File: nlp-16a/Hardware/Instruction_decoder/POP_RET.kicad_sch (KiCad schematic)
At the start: 12 parts

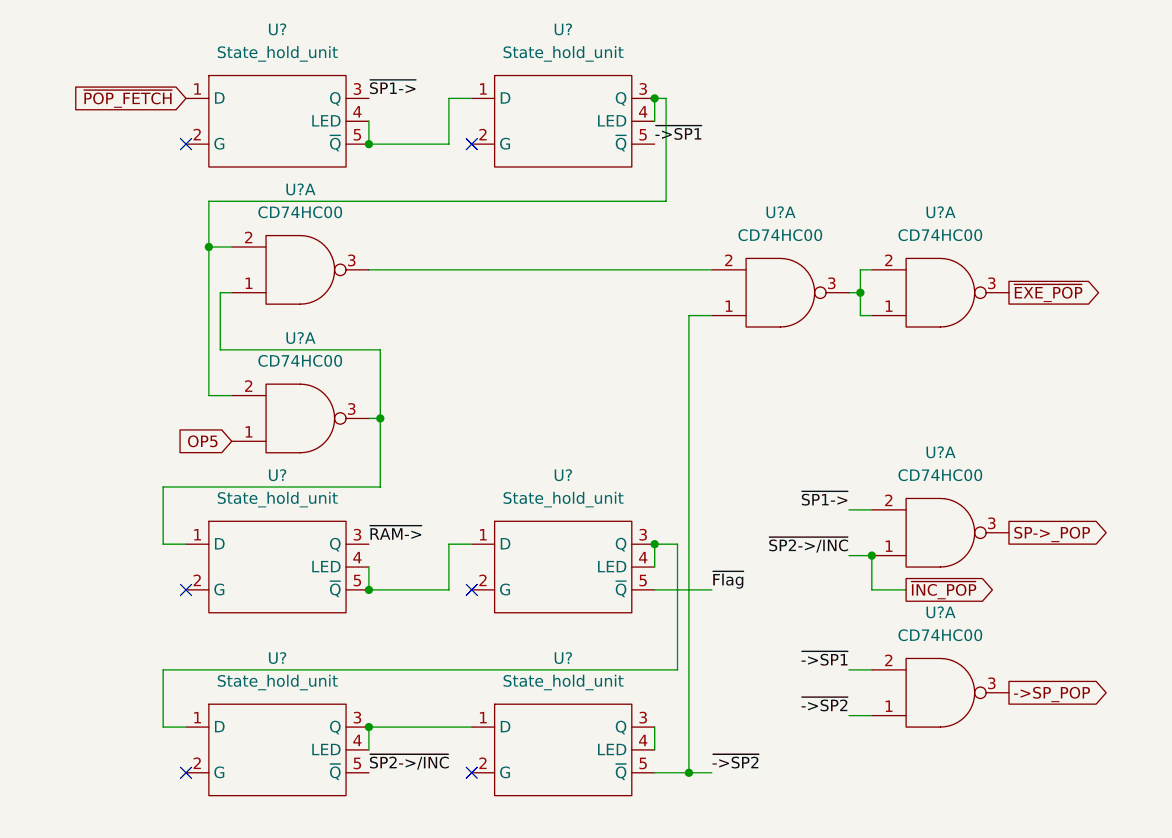
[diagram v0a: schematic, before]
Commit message: 命令デコーダ ロジック部の設計だいたい完了git statusgit statusやったぜ
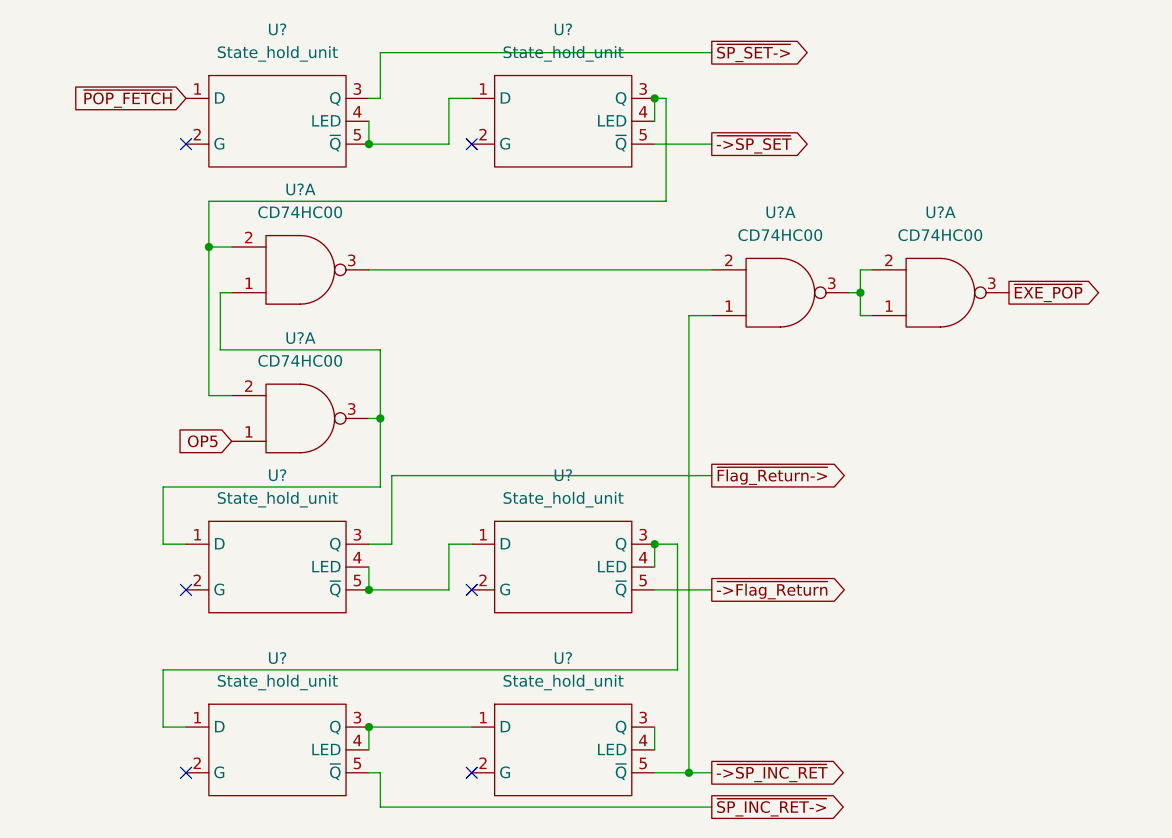
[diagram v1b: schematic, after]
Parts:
- removed U? (x2): CD74HC00, Package_DIP:DIP-14_W7.62mm, symbol CD74HCXX:CD74HC00
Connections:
- net ~{->SP1} renamed ~{->SP_SET}
- net ~{->SP2} renamed ~{->SP_INC_RET}
- net ~{Flag} renamed ~{->Flag_Return}
- net ~{INC_POP} renamed ~{SP_INC_RET->}
- net ~{RAM->} renamed ~{Flag_Return->}
- net ~{SP1->} renamed ~{SP_SET->}
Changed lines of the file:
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@@
   (junction (at 165.1 53.34) (diameter 0) (color 0 0 0 0)
-  )
-  (junction (at 166.37 82.55) (diameter 0) (color 0 0 0 0)
   )
   (junction (at 142.24 31.75) (diameter 0) (color 0 0 0 0)
@@
   (no_connect (at 121.92 86.36))
   (no_connect (at 90.17 106.68))
-  (wire (pts (xy 166.37 82.55) (xy 166.37 86.36))
+  (wire (pts (xy 142.24 36.83) (xy 148.59 36.83))
     (stroke (width 0) (type default) (color 0 0 0 0))
   )
@@
     (stroke (width 0) (type default) (color 0 0 0 0))
   )
+  (wire (pts (xy 113.03 73.66) (xy 148.59 73.66))
+    (stroke (width 0) (type default) (color 0 0 0 0))
+  )
   (wire (pts (xy 146.05 55.88) (xy 148.59 55.88))
     (stroke (width 0) (type default) (color 0 0 0 0))
@@
     (stroke (width 0) (type default) (color 0 0 0 0))
   )
+  (wire (pts (xy 111.76 31.75) (xy 111.76 26.67))
+    (stroke (width 0) (type default) (color 0 0 0 0))
+  )
   (wire (pts (xy 142.24 81.28) (xy 144.78 81.28))
     (stroke (width 0) (type default) (color 0 0 0 0))
@@
     (stroke (width 0) (type default) (color 0 0 0 0))
   )
+  (wire (pts (xy 110.49 31.75) (xy 111.76 31.75))
+    (stroke (width 0) (type default) (color 0 0 0 0))
+  )
   (wire (pts (xy 143.51 43.18) (xy 92.71 43.18))
     (stroke (width 0) (type default) (color 0 0 0 0))
@@
     (stroke (width 0) (type default) (color 0 0 0 0))
   )
+  (wire (pts (xy 111.76 106.68) (xy 111.76 110.49))
+    (stroke (width 0) (type default) (color 0 0 0 0))
+  )
   (wire (pts (xy 142.24 101.6) (xy 142.24 104.14))
     (stroke (width 0) (type default) (color 0 0 0 0))
@@
     (stroke (width 0) (type default) (color 0 0 0 0))
   )
-  (wire (pts (xy 163.83 82.55) (xy 166.37 82.55))
-    (stroke (width 0) (type default) (color 0 0 0 0))
-  )
-  (wire (pts (xy 170.18 86.36) (xy 166.37 86.36))
+  (wire (pts (xy 113.03 81.28) (xy 113.03 73.66))
+    (stroke (width 0) (type default) (color 0 0 0 0))
+  )
+  (wire (pts (xy 111.76 110.49) (xy 148.59 110.49))
     (stroke (width 0) (type default) (color 0 0 0 0))
   )
@@
     (stroke (width 0) (type default) (color 0 0 0 0))
   )
-  (wire (pts (xy 163.83 77.47) (xy 166.37 77.47))
+  (wire (pts (xy 110.49 106.68) (xy 111.76 106.68))
+    (stroke (width 0) (type default) (color 0 0 0 0))
+  )
+  (wire (pts (xy 110.49 81.28) (xy 113.03 81.28))
     (stroke (width 0) (type default) (color 0 0 0 0))
   )
@@
     (stroke (width 0) (type default) (color 0 0 0 0))
   )
+  (wire (pts (xy 111.76 26.67) (xy 148.59 26.67))
+    (stroke (width 0) (type default) (color 0 0 0 0))
+  )
   (wire (pts (xy 90.17 101.6) (xy 87.63 101.6))
     (stroke (width 0) (type default) (color 0 0 0 0))
@@
     (stroke (width 0) (type default) (color 0 0 0 0))
   )
-  (wire (pts (xy 163.83 95.25) (xy 166.37 95.25))
-    (stroke (width 0) (type default) (color 0 0 0 0))
-  )
   (wire (pts (xy 143.51 31.75) (xy 143.51 43.18))
     (stroke (width 0) (type default) (color 0 0 0 0))
@@
     (stroke (width 0) (type default) (color 0 0 0 0))
   )
-  (wire (pts (xy 163.83 100.33) (xy 166.37 100.33))
-    (stroke (width 0) (type default) (color 0 0 0 0))
-  )
   (wire (pts (xy 163.83 53.34) (xy 165.1 53.34))
     (stroke (width 0) (type default) (color 0 0 0 0))
@@
     (stroke (width 0) (type default) (color 0 0 0 0))
   )
-  (label "~{SP1->}" (at 163.83 77.47 180)
-    (effects (font (size 1.27 1.27)) (justify right bottom))
-  )
-  (label "~{->SP1}" (at 163.83 95.25 180)
-    (effects (font (size 1.27 1.27)) (justify right bottom))
-  )
-  (label "~{SP2->{slash}INC}" (at 110.49 106.68 0)
-    (effects (font (size 1.27 1.27)) (justify left bottom))
-  )
-  (label "~{->SP2}" (at 163.83 100.33 180)
-    (effects (font (size 1.27 1.27)) (justify right bottom))
-  )
-  (label "~{SP2->{slash}INC}" (at 163.83 82.55 180)
-    (effects (font (size 1.27 1.27)) (justify right bottom))
-  )
-  (label "~{SP1->}" (at 110.49 31.75 0)
-    (effects (font (size 1.27 1.27)) (justify left bottom))
-  )
-  (label "~{RAM->}" (at 110.49 81.28 0)
-    (effects (font (size 1.27 1.27)) (justify left bottom))
-  )
-  (label "~{->SP1}" (at 142.24 36.83 0)
-    (effects (font (size 1.27 1.27)) (justify left bottom))
-  )
-  (label "~{Flag}" (at 148.59 86.36 0)
-    (effects (font (size 1.27 1.27)) (justify left bottom))
-  )
-  (label "~{->SP2}" (at 148.59 106.68 0)
-    (effects (font (size 1.27 1.27)) (justify left bottom))
-  )
   (global_label "~{EXE_POP}" (shape output) (at 181.61 53.34 0) (fields_autoplaced)
     (effects (font (size 1.27 1.27)) (justify left))
     (property "Intersheet References" "${INTERSHEET_REFS}" (id 0) (at 192.3688 53.2606 0)
+      (effects (font (size 1.27 1.27)) (justify left) hide)
+    )
+  )
+  (global_label "~{SP_INC_RET->}" (shape output) (at 148.59 110.49 0) (fields_autoplaced)
+    (effects (font (size 1.27 1.27)) (justify left))
+    (property "Intersheet References" "${INTERSHEET_REFS}" (id 0) (at 165.1545 110.4106 0)
       (effects (font (size 1.27 1.27)) (justify left) hide)
     )
@@
     )
   )
-  (global_label "SP->_POP" (shape output) (at 181.61 80.01 0) (fields_autoplaced)
-    (effects (font (size 1.27 1.27)) (justify left))
-    (property "Intersheet References" "${INTERSHEET_REFS}" (id 0) (at 194.4855 79.9306 0)
+  (global_label "~{->SP_INC_RET}" (shape output) (at 148.59 106.68 0) (fields_autoplaced)
+    (effects (font (size 1.27 1.27)) (justify left))
+    (property "Intersheet References" "${INTERSHEET_REFS}" (id 0) (at 165.1545 106.6006 0)
+      (effects (font (size 1.27 1.27)) (justify left) hide)
+    )
+  )
+  (global_label "~{SP_SET->}" (shape output) (at 148.59 26.67 0) (fields_autoplaced)
+    (effects (font (size 1.27 1.27)) (justify left))
+    (property "Intersheet References" "${INTERSHEET_REFS}" (id 0) (at 160.9212 26.5906 0)
+      (effects (font (size 1.27 1.27)) (justify left) hide)
+    )
+  )
+  (global_label "~{->SP_SET}" (shape output) (at 148.59 36.83 0) (fields_autoplaced)
+    (effects (font (size 1.27 1.27)) (justify left))
+    (property "Intersheet References" "${INTERSHEET_REFS}" (id 0) (at 160.9212 36.7506 0)
       (effects (font (size 1.27 1.27)) (justify left) hide)
     )
@@
     )
   )
-  (global_label "->SP_POP" (shape output) (at 181.61 97.79 0) (fields_autoplaced)
-    (effects (font (size 1.27 1.27)) (justify left))
-    (property "Intersheet References" "${INTERSHEET_REFS}" (id 0) (at 194.4855 97.7106 0)
-      (effects (font (size 1.27 1.27)) (justify left) hide)
-    )
-  )
-  (global_label "~{INC_POP}" (shape output) (at 170.18 86.36 0) (fields_autoplaced)
-    (effects (font (size 1.27 1.27)) (justify left))
-    (property "Intersheet References" "${INTERSHEET_REFS}" (id 0) (at 180.6364 86.2806 0)
+  (global_label "~{Flag_Return->}" (shape output) (at 148.59 73.66 0) (fields_autoplaced)
+    (effects (font (size 1.27 1.27)) (justify left))
+    (property "Intersheet References" "${INTERSHEET_REFS}" (id 0) (at 165.336 73.5806 0)
+      (effects (font (size 1.27 1.27)) (justify left) hide)
+    )
+  )
+  (global_label "~{->Flag_Return}" (shape output) (at 148.59 86.36 0) (fields_autoplaced)
+    (effects (font (size 1.27 1.27)) (justify left))
+    (property "Intersheet References" "${INTERSHEET_REFS}" (id 0) (at 165.336 86.2806 0)
       (effects (font (size 1.27 1.27)) (justify left) hide)
     )
@@
     (pin "14")
     (pin "7")
-    (pin "1")
-    (pin "2")
-    (pin "3")
-    (pin "4")
-    (pin "5")
-    (pin "6")
-    (pin "10")
-    (pin "8")
-    (pin "9")
-    (pin "11")
-    (pin "12")
-    (pin "13")
-  )
-  (symbol (lib_id "CD74HCXX:CD74HC00") (at 173.99 80.01 0) (mirror x) (unit 1)
-    (in_bom yes) (on_board yes)
-    (property "Reference" "U?" (id 0) (at 173.99 71.12 0))
-    (property "Value" "CD74HC00" (id 1) (at 173.99 73.66 0))
-    (property "Footprint" "Package_DIP:DIP-14_W7.62mm" (id 2) (at 173.99 86.36 0)
-      (effects (font (size 1.27 1.27)) hide)
-    )
-    (property "Datasheet" "" (id 3) (at 168.91 80.01 0))
-    (pin "14")
-    (pin "7")
-    (pin "1")
-    (pin "2")
-    (pin "3")
-    (pin "4")
-    (pin "5")
-    (pin "6")
-    (pin "10")
-    (pin "8")
-    (pin "9")
-    (pin "11")
-    (pin "12")
-    (pin "13")
-  )
-  (symbol (lib_id "CD74HCXX:CD74HC00") (at 173.99 97.79 0) (mirror x) (unit 1)
-    (in_bom yes) (on_board yes)
-    (property "Reference" "U?" (id 0) (at 173.99 88.9 0))
-    (property "Value" "CD74HC00" (id 1) (at 173.99 91.44 0))
-    (property "Footprint" "Package_DIP:DIP-14_W7.62mm" (id 2) (at 173.99 104.14 0)
-      (effects (font (size 1.27 1.27)) hide)
-    )
-    (property "Datasheet" "" (id 3) (at 168.91 97.79 0))
-    (pin "14")
-    (pin "7")
